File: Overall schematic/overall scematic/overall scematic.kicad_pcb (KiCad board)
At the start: 2 copper layers, 31 parts, among them IC1 battery protection IC DW01A-G, J1 USB_B_Micro, J10 Conn_01x02_Pin, J11 Conn_01x02_Pin, J2 Conn_01x02_Pin, J3 Battery Charger IC TP4056, J4 Conn_01x02_Pin, J5 Conn_01x02_Pin, J6 Conn_01x02_Pin, J8 DB25_Receptacle, J9 DB25_Receptacle, Q1 Dual Mosfet FS8205A, U1 Voltage Regulator HT75xx-1-SO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, U2 AT24CS01-STUM, U4 HDC1080, U5 MCP9701AT-E_TT

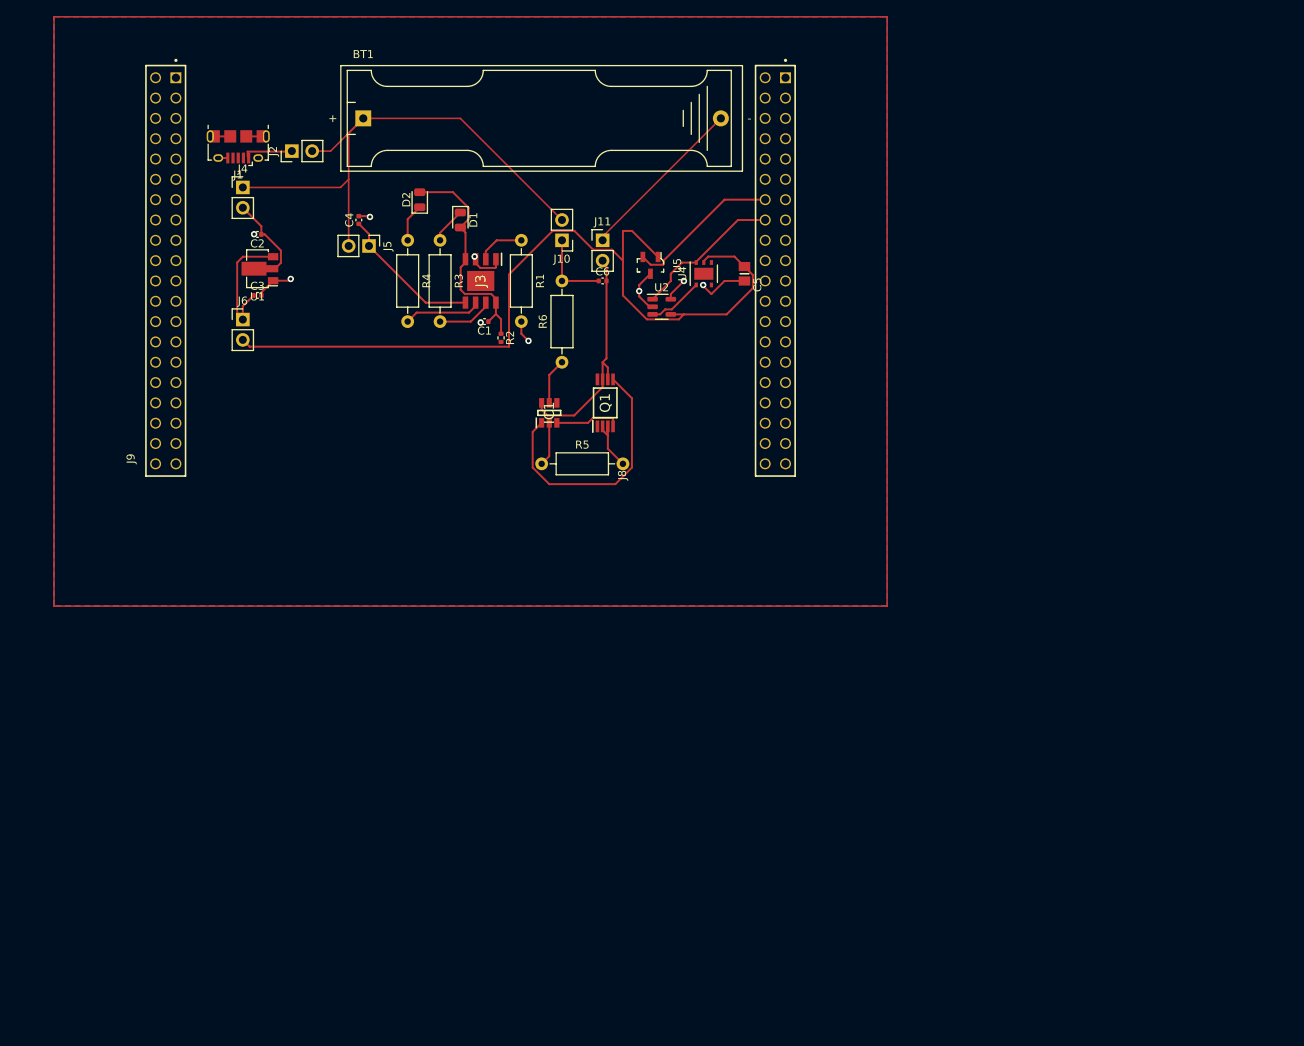
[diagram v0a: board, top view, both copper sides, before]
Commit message: The final Gerber
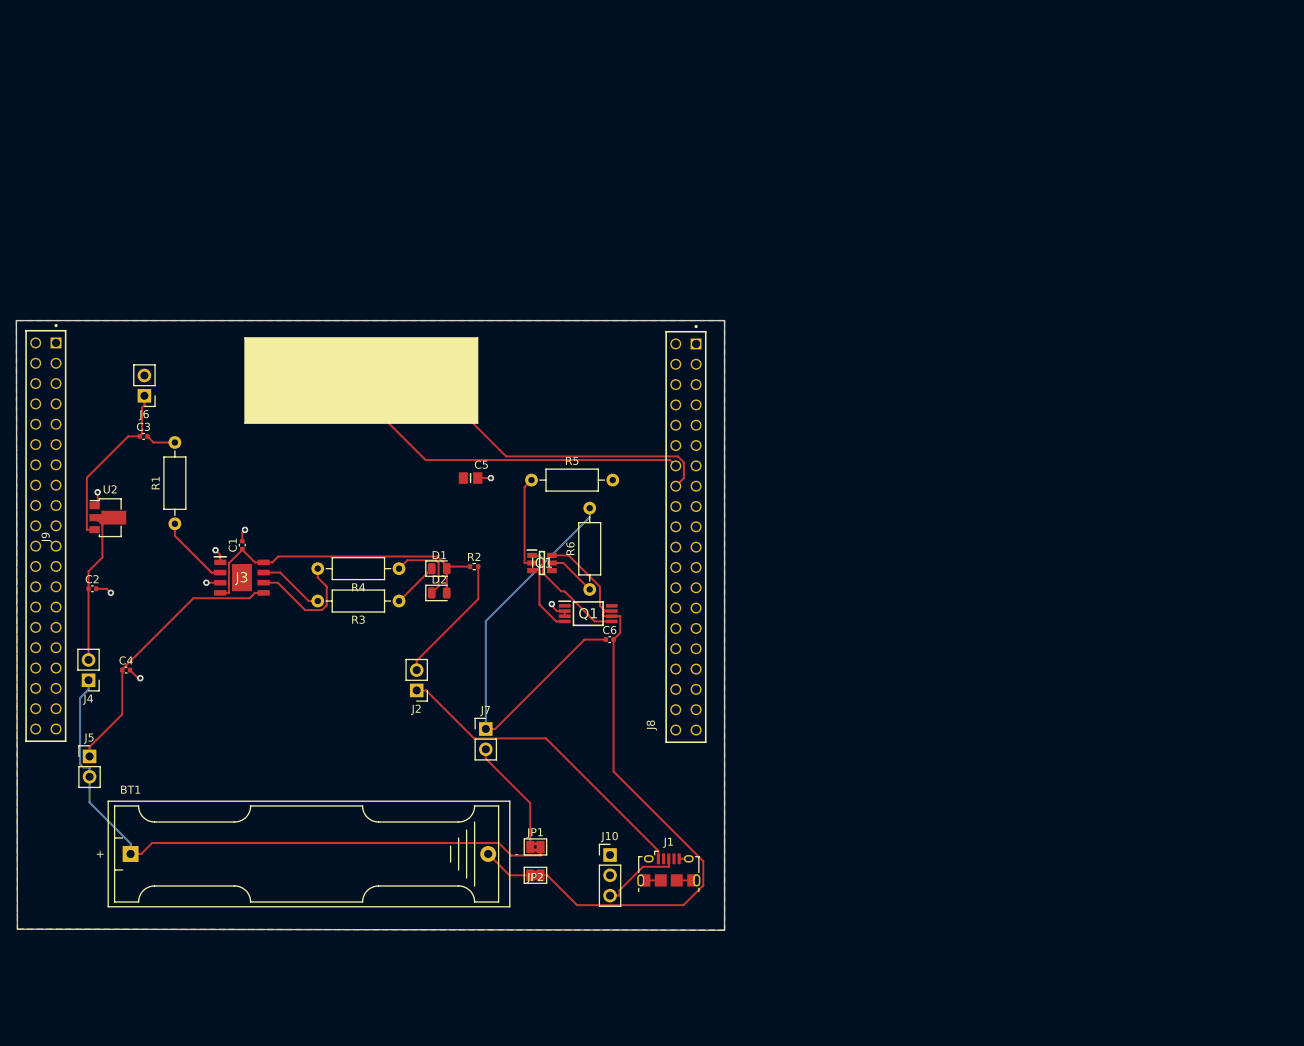
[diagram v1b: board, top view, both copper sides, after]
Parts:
- removed J11: Conn_01x02_Pin, Connector_PinHeader_2.54mm:PinHeader_1x02_P2.54mm_Vertical
- added J7: Conn_01x02_Pin, Connector_PinHeader_2.54mm:PinHeader_1x02_P2.54mm_Vertical, F.Cu at (109.9, 114.4)
- added JP1: Jumper_2_Bridged, Jumper:SolderJumper-2_P1.3mm_Bridged2Bar_Pad1.0x1.5mm, F.Cu at (116.1, 129.2)
- added JP2: Jumper_2_Bridged, Jumper:SolderJumper-2_P1.3mm_Bridged2Bar_Pad1.0x1.5mm, F.Cu at (116.1, 132.7)
- C1, C2, C3, C4, C6: value 10uf -> C
- D1: value Green LED -> LED
- D2: value Red LED -> LED
- IC1: value battery protection IC DW01A-G -> DW01A-G; footprint DW01A:SOT95P280X135-6N -> BAT60JFILM:DW01A
- J10: value Conn_01x02_Pin -> Conn_01x09_Pin; footprint Connector_PinHeader_2.54mm:PinHeader_1x02_P2.54mm_Vertical -> Connector_PinHeader_2.54mm:PinHeader_1x03_P2.54mm_Vertical
- J3: value Battery Charger IC TP4056 -> TP4056; footprint TP4056:SOIC127P600X175-9N -> BAT60JFILM:TP4056
- Q1: value Dual Mosfet FS8205A -> FS8205A; footprint FB8205A:SOP65P640X120-8N -> BAT60JFILM:FB8205A
- R1: value 1.6k -> R
- R2: value 400m -> R
- R3, R4, R5: value 1k -> R
- R6: value 100 -> R
- U1: value Voltage Regulator HT75xx-1-SOT89 -> HDC1080; footprint Package_TO_SOT_SMD:SOT-89-3 -> Package_SON:Texas_PWSON-N6
- U2: value AT24CS01-STUM -> HT75xx-1-SOT89; footprint Package_TO_SOT_SMD:SOT-23-5 -> Package_TO_SOT_SMD:SOT-89-3
- U4: value HDC1080 -> AT24CS01-STUM; footprint Package_SON:Texas_PWSON-N6 -> Package_TO_SOT_SMD:SOT-23-5
- moved J1 105.2 mm to (132.7, 132.1), turned to 0 degrees
- moved BT1 96.4 mm to (65.5, 130.0)
- moved J10 77.1 mm to (125.4, 130.2), turned to 0 degrees
- moved U2 73.8 mm to (62.9, 88.0)
- moved J5 72.7 mm to (60.3, 117.9), turned to 0 degrees
- moved J2 69.2 mm to (101.2, 109.6), turned to 180 degrees
- moved J4 64.5 mm to (60.2, 108.3), turned to 180 degrees
- moved C4 63.3 mm to (64.9, 107.1), turned to 0 degrees
- moved R1 56.0 mm to (71.0, 88.8), turned to 90 degrees
- moved U4 50.4 mm to (88.3, 70.1), turned to 180 degrees
- moved D2 49.2 mm to (104.0, 97.4), turned to 0 degrees
- moved C2 48.9 mm to (60.7, 96.9), turned to 0 degrees
- moved J3 47.6 mm to (79.4, 95.5), turned to 0 degrees
- moved R3 45.4 mm to (99.0, 98.4), turned to 180 degrees
- moved C6 44.8 mm to (125.3, 103.3)
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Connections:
- net ADC renamed /Micro controller pin outs/Analogue_out
- net Net-(J1-VBUS) renamed Vreg_Out
- C6 pad 1: Net-(J10-Pin_1) -> Net-(J7-Pin_1)
- J10 pad 1: Net-(J10-Pin_1) -> /Supply_Voltage
- J10 pad 2: /Battery+ -> /Supply_Voltage
- J2 pad 2: /Battery+ -> /Power module/VCC
- J8 pad 10: GND -> /Micro controller pin outs/NRST
- J8 pad 12: GND -> /Micro controller pin outs/PB6
- J8 pad 13: GND -> /Micro controller pin outs/PA0
- J8 pad 15: SPI -> GND
- J8 pad 25: GND -> /Micro controller pin outs/PB7
- J9 pad 11: USART2 -> GND
- J9 pad 23: USART1 -> GND
- R2 pad 2: +5V -> /Power module/VCC
- R6 pad 2: Net-(J10-Pin_1) -> Net-(J7-Pin_1)
- U1 pad 1: GND -> /SDA
- U1 pad 2: Net-(J4-Pin_2) -> GND
- U1 pad 3: Net-(J6-Pin_1) -> unconnected-(U1-NC-Pad3)
- U2 pad 1: /SCL -> GND
- U2 pad 2: GND -> Net-(J4-Pin_2)
- U2 pad 3: /SDA -> Net-(J6-Pin_1)
- U4 pad 1: /SDA -> /SCL
- U4 pad 3: unconnected-(U4-NC-Pad3) -> /SDA
- U4 pad 4: unconnected-(U4-NC-Pad4) -> /Supply_Voltage
- U4 pad 5: /Supply_Voltage -> GND
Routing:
- net /Supply_Voltage: track 104.4 -> 8.92 mm, vias 0 -> 2
- net Net-(J7-Pin_1): track 0.00 -> 52.6 mm
- net Net-(IC1-GND): track 28.9 -> 76.2 mm
- net /SCL: track 18.8 -> 57.3 mm
- net Vreg_Out: track 6.20 -> 39.5 mm
- net /Micro controller pin outs/Analogue_out: track 19.3 -> 44.7 mm
- net /Power module/OD: track 32.2 -> 14.4 mm
- net /Power module/VCC: track 0.00 -> 16.1 mm
- net Net-(J3-BAT): track 18.3 -> 34.2 mm
- net /Battery-: track 21.4 -> 6.36 mm
- net /Power module/V_Battery: track 0.00 -> 14.5 mm
- net /Power module/Vcc_IC: track 28.9 -> 40.6 mm
- net /Battery+: track 68.5 -> 78.8 mm
- net Data +: track 0.00 -> 10.2 mm
- net Net-(J10-Pin_1): track 9.68 -> 0.00 mm
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- added copper zone on F.Cu, net /Supply_Voltage
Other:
- board outline added: 88.5 x 76.2 mm

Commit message: hail mary
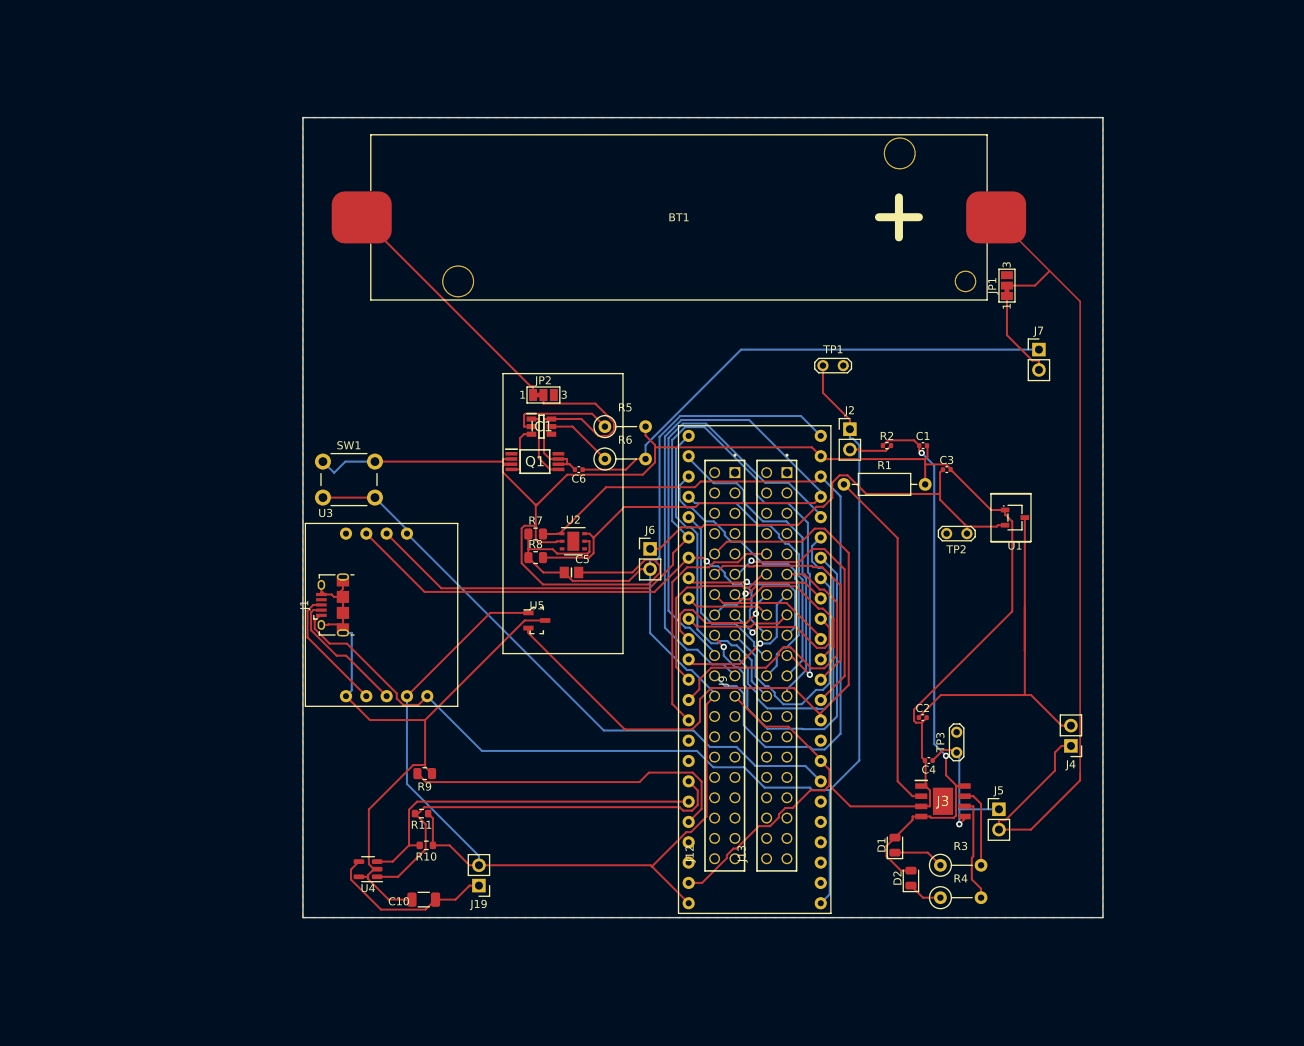
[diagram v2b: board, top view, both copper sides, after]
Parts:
- removed J10: Conn_01x09_Pin, Connector_PinHeader_2.54mm:PinHeader_1x03_P2.54mm_Vertical
- removed J8: DB25_Receptacle, SSQ-120-03-G-D:SAMTEC_SSQ-120-03-G-D
- added C10: 10nF, Capacitor_SMD:C_1206_3216Metric, F.Cu at (102.1, 135.8)
- added J12: Conn_01x24_Socket, BAT60JFILM:SAMTEC_SSQ-120-03-G-D, F.Cu at (139.7, 106.5)
- added J13: Conn_01x24_Socket, BAT60JFILM:SAMTEC_SSQ-120-03-G-D, F.Cu at (146.2, 106.5)
- added J19: Conn_01x02_Pin, Connector_PinHeader_2.54mm:PinHeader_1x02_P2.54mm_Vertical, F.Cu at (109.0, 134.0)
- added R10: 1k, Resistor_SMD:R_0603_1608Metric, F.Cu at (102.4, 129.0)
- added R11: 1k, Resistor_SMD:R_0603_1608Metric, F.Cu at (101.8, 125.0)
- added R7: 4.7k, Resistor_SMD:R_0805_2012Metric, F.Cu at (116.1, 90.0)
- added R8: 4.7k, Resistor_SMD:R_0805_2012Metric, F.Cu at (116.1, 93.0)
- added R9: 10k, Resistor_SMD:R_0805_2012Metric, F.Cu at (102.2, 120.0)
- added SW1: SW_Push, Button_Switch_THT:SW_PUSH_6mm, F.Cu at (89.5, 81.0)
- added TP1: TestPoint, TestPoint:TestPoint_2Pads_Pitch2.54mm_Drill0.8mm, F.Cu at (152.0, 69.0)
- added TP2: TestPoint, TestPoint:TestPoint_2Pads_Pitch2.54mm_Drill0.8mm, F.Cu at (170.0, 90.0)
- added TP3: TestPoint, TestPoint:TestPoint_2Pads_Pitch2.54mm_Drill0.8mm, F.Cu at (168.7, 117.4)
- added U3: STLINK_UCT, BAT60JFILM:STLINK_UCT, F.Cu at (96.2, 100.2)
- BT1: footprint Battery:BatteryHolder_Keystone_2466_1xAAA -> BAT60JFILM:18650_Holder_SMD
- C1, C4, C6: value C -> 10uf
- C2, C3: value C -> 1uf
- C5: footprint CL21B104KCFNNNE:CAPC2012X140N -> BAT60JFILM:CAPC2012X140N
- D1: value LED -> Green LED
- D2: value LED -> Red LED
- IC1: value DW01A-G -> battery protection IC DW01A-G
- J3: value TP4056 -> Battery Charger IC TP4056
- J9: value DB25_Receptacle -> Conn_02x24_Counter_Clockwise; footprint SSQ-120-03-G-D:SAMTEC_SSQ-120-03-G-D -> BAT60JFILM:STM32F051C6T6
- JP1, JP2: footprint Jumper:SolderJumper-2_P1.3mm_Bridged2Bar_Pad1.0x1.5mm -> Jumper:SolderJumper-3_P1.3mm_Bridged12_Pad1.0x1.5mm_NumberLabels
- Q1: value FS8205A -> Dual Mosfet FS8205A
- R1: value R -> 1.6k
- R2: value R -> 400m
- R3, R4, R5: value R -> 1k; footprint Resistor_THT:R_Axial_DIN0207_L6.3mm_D2.5mm_P10.16mm_Horizontal -> Resistor_THT:R_Axial_DIN0207_L6.3mm_D2.5mm_P5.08mm_Vertical
- R6: value R -> 100; footprint Resistor_THT:R_Axial_DIN0207_L6.3mm_D2.5mm_P10.16mm_Horizontal -> Resistor_THT:R_Axial_DIN0207_L6.3mm_D2.5mm_P5.08mm_Vertical
- U1: value HDC1080 -> MCP1700T-3302E_TT; footprint Package_SON:Texas_PWSON-N6 -> BAT60JFILM:SOT-23-3_L2.9-W1.6-P1.90-LS2.8-BR
- U2: value HT75xx-1-SOT89 -> HDC1080; footprint Package_TO_SOT_SMD:SOT-89-3 -> Package_SON:Texas_PWSON-N6
- U5: footprint MCP9701AT-E_TT:SOT-23-3 -> BAT60JFILM:SOT-23-3
- moved J4 123.1 mm to (183.0, 116.5)
- moved J5 113.9 mm to (174.0, 124.5)
- moved C2 105.0 mm to (164.5, 113.0)
- moved BT1 104.6 mm to (134.0, 51.0)
- moved C4 101.0 mm to (165.2, 118.4), turned to 180 degrees
- moved C3 100.5 mm to (167.5, 82.0)
- moved J9 92.5 mm to (145.6, 108.2)
- moved J3 92.0 mm to (167.0, 123.5)
- moved JP1 91.6 mm to (175.0, 59.0), turned to 90 degrees
- moved C1 86.0 mm to (164.5, 79.0), turned to 0 degrees
- moved J7 83.8 mm to (179.0, 67.0)
- moved R1 83.8 mm to (154.6, 83.8), turned to 0 degrees
- moved R4 79.2 mm to (166.7, 135.5), turned to 0 degrees
- moved U1 76.8 mm to (176.0, 88.0), turned to 180 degrees
- moved R3 75.3 mm to (166.7, 131.5), turned to 0 degrees
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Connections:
- net /Power module/VCC renamed /Power module/5V
- J9 pad 10: GND -> /Micro controller pin outs/PA0
- J9 pad 11: GND -> /Micro controller pin outs/PA1
- J9 pad 12: I2C2 -> /Micro controller pin outs/PA2
- J9 pad 13: GND -> /Micro controller pin outs/PA3
- J9 pad 14: GND -> /Micro controller pin outs/PA4
- J9 pad 15: GND -> /Micro controller pin outs/PA5
- J9 pad 16: GND -> /Micro controller pin outs/PA6
- J9 pad 17: GND -> /Micro controller pin outs/PA7
- J9 pad 18: GND -> /Micro controller pin outs/PB0
- J9 pad 19: GND -> /Micro controller pin outs/PB1
- J9 pad 20: GND -> /Micro controller pin outs/PB2
- J9 pad 21: GND -> /SCL
- J9 pad 22: GND -> /SDA
- J9 pad 24: I2C1 -> /Supply_Voltage
- J9 pad 25: GND -> /Micro controller pin outs/PB12
- J9 pad 26: (no net) -> /Micro controller pin outs/PB13
- J9 pad 27: (no net) -> /Micro controller pin outs/PB14
- J9 pad 28: (no net) -> /Micro controller pin outs/PB15
- J9 pad 29: (no net) -> /Micro controller pin outs/PA8
- J9 pad 30: (no net) -> /Micro controller pin outs/PA9
- J9 pad 31: (no net) -> /Micro controller pin outs/PA10
- J9 pad 32: (no net) -> /Micro controller pin outs/PA11
- J9 pad 33: (no net) -> /Micro controller pin outs/PA12
- J9 pad 34: (no net) -> /Micro controller pin outs/PA13
- J9 pad 35: (no net) -> /Micro controller pin outs/PF6
- J9 pad 36: (no net) -> /Micro controller pin outs/PF7
- J9 pad 37: (no net) -> /Micro controller pin outs/PA14
- J9 pad 38: (no net) -> /Micro controller pin outs/PA15
- J9 pad 39: (no net) -> /Micro controller pin outs/PB3
- J9 pad 40: (no net) -> /Micro controller pin outs/PB4
- U1 pad 1: /SDA -> GND
- U1 pad 2: GND -> Net-(J6-Pin_1)
- U1 pad 3: unconnected-(U1-NC-Pad3) -> Net-(J4-Pin_2)
- U2 pad 1: GND -> /SDA
- U2 pad 2: Net-(J4-Pin_2) -> GND
- U2 pad 3: Net-(J6-Pin_1) -> unconnected-(U2-NC-Pad3)
- U4 pad 1: /SCL -> /Micro controller pin outs/PB6
- U4 pad 3: /SDA -> /Micro controller pin outs/PB7
- U4 pad 4: /Supply_Voltage -> Net-(J19-Pin_1)
- U5 pad 2: /Micro controller pin outs/Analogue_out -> /Micro controller pin outs/PA0
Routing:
- net GND: track 32.7 -> 339.8 mm, vias 10 -> 0
- net /Supply_Voltage: track 8.92 -> 197.6 mm, vias 2 -> 0
- net Vreg_Out: track 39.5 -> 147.4 mm
- net /Micro controller pin outs/PA9: track 0.00 -> 103.8 mm, vias 0 -> 1
- net /Micro controller pin outs/PA0: track 0.00 -> 89.3 mm
- net /SDA: track 11.3 -> 93.9 mm
- net /Micro controller pin outs/NRST: track 0.43 -> 77.2 mm
- net /Micro controller pin outs/PA10: track 0.00 -> 61.3 mm, vias 0 -> 1
- net /Micro controller pin outs/PB2: track 0.00 -> 54.7 mm
- net /Micro controller pin outs/PB6: track 0.00 -> 52.0 mm
- net /Micro controller pin outs/PB7: track 0.00 -> 46.0 mm
- net /Micro controller pin outs/Analogue_out: track 44.7 -> 0.00 mm
- net /Micro controller pin outs/PB0: track 0.00 -> 44.7 mm, vias 0 -> 1
- net Net-(IC1-GND): track 76.2 -> 32.2 mm
- net /Micro controller pin outs/BOOT: track 0.00 -> 43.8 mm
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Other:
- board size 88.5 x 76.2 mm -> 100 x 100 mm
